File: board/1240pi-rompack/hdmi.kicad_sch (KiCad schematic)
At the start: 3 parts, among them J2 RaspberryPi_CM4_B, J3 HDMI_A, J4 HDMI_A

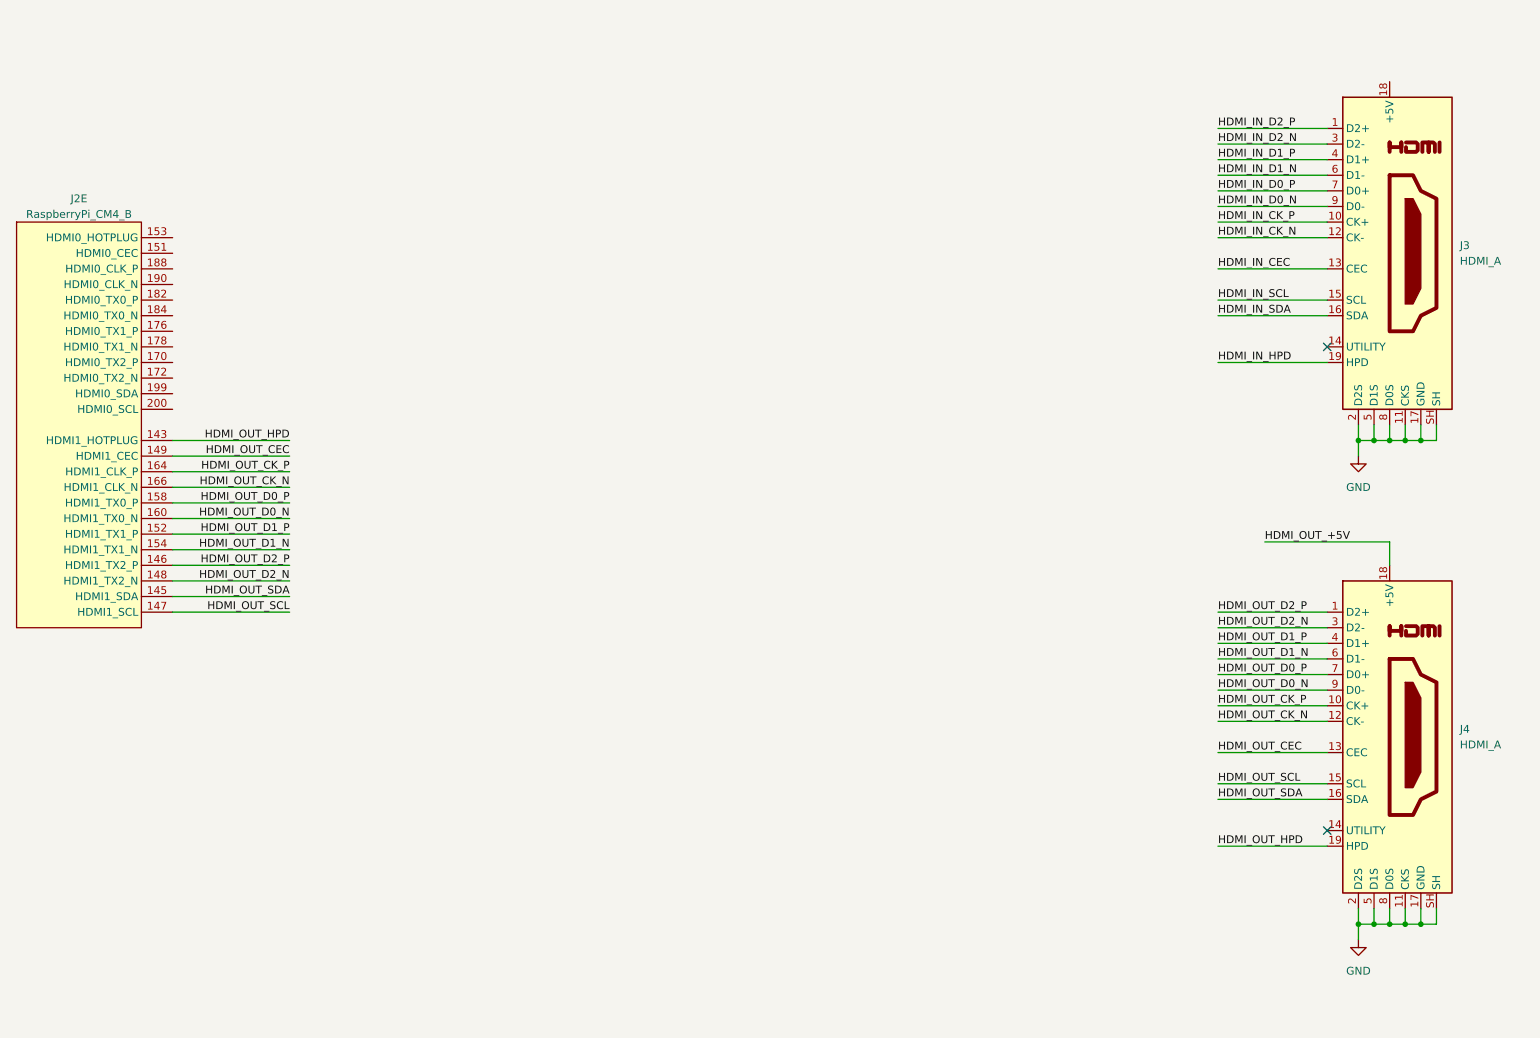
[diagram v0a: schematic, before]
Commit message: Route HDMI output port.
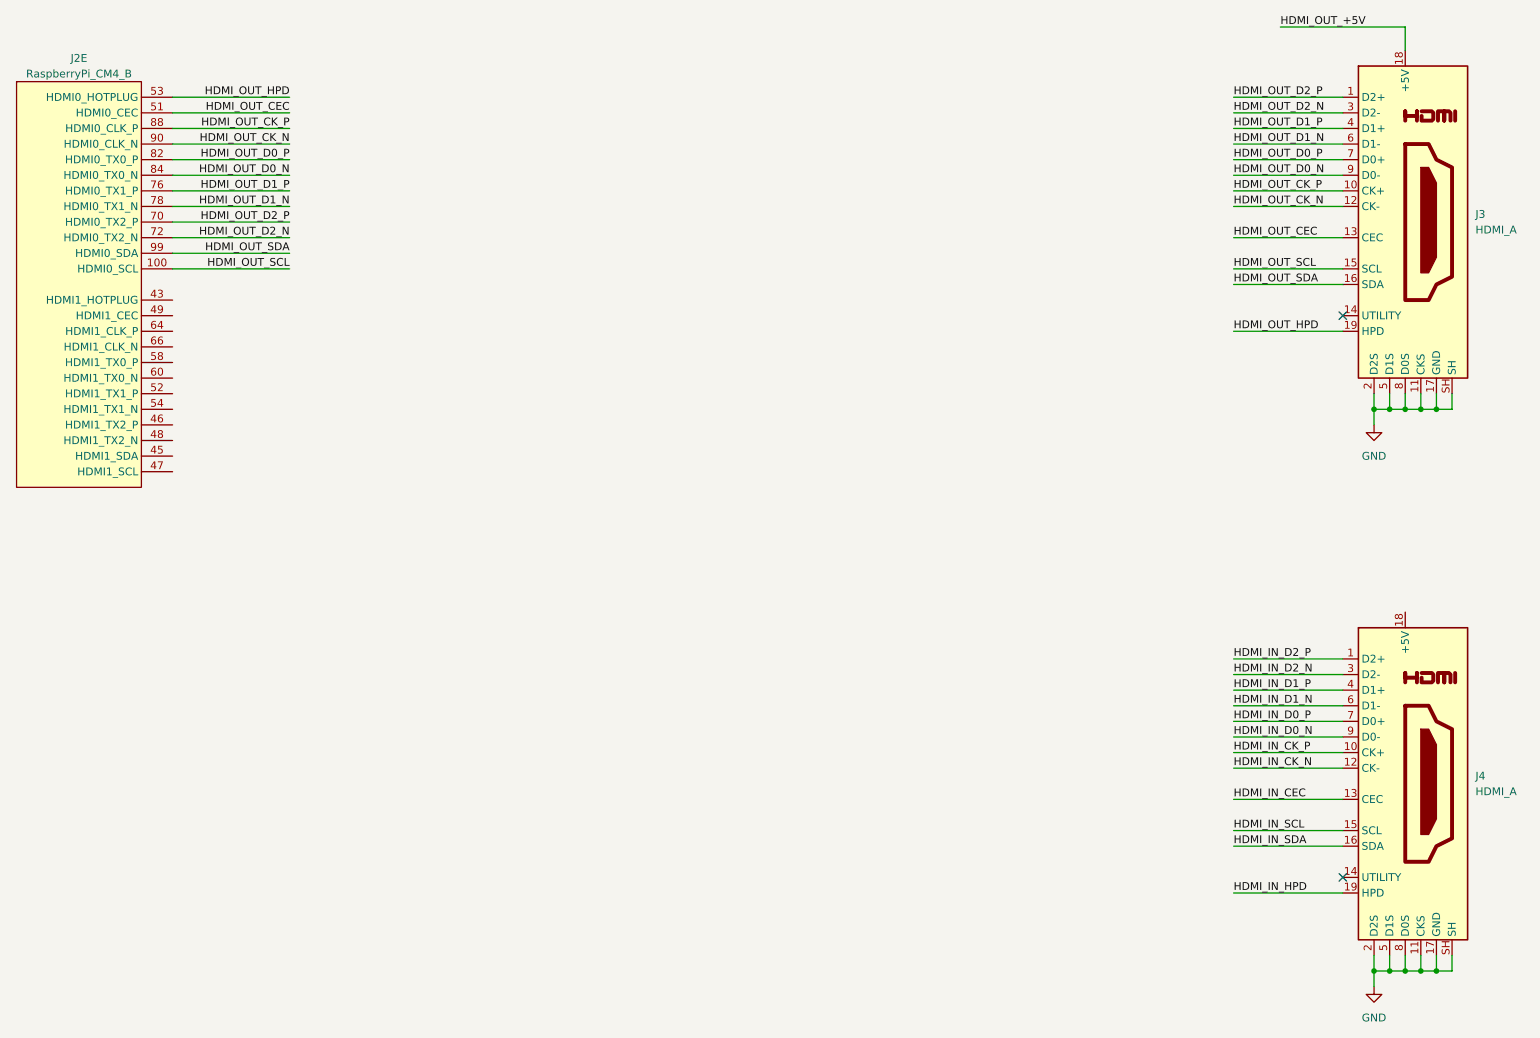
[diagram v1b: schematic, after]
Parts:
- renumbered J4 to J3, J3 to J4
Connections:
- net HDMI_OUT_CEC: now also J2.51 (HDMI0_CEC); no longer J2.149 (HDMI1_CEC)
- net HDMI_OUT_CK_N: now also J2.90 (HDMI0_CLK_N); no longer J2.166 (HDMI1_CLK_N)
- net HDMI_OUT_CK_P: now also J2.88 (HDMI0_CLK_P); no longer J2.164 (HDMI1_CLK_P)
- net HDMI_OUT_D0_N: now also J2.84 (HDMI0_TX0_N); no longer J2.160 (HDMI1_TX0_N)
- net HDMI_OUT_D0_P: now also J2.82 (HDMI0_TX0_P); no longer J2.158 (HDMI1_TX0_P)
- net HDMI_OUT_D1_N: now also J2.78 (HDMI0_TX1_N); no longer J2.154 (HDMI1_TX1_N)
- net HDMI_OUT_D1_P: now also J2.76 (HDMI0_TX1_P); no longer J2.152 (HDMI1_TX1_P)
- net HDMI_OUT_D2_N: now also J2.72 (HDMI0_TX2_N); no longer J2.148 (HDMI1_TX2_N)
- net HDMI_OUT_D2_P: now also J2.70 (HDMI0_TX2_P); no longer J2.146 (HDMI1_TX2_P)
- net HDMI_OUT_HPD: now also J2.53 (HDMI0_HOTPLUG); no longer J2.143 (HDMI1_HOTPLUG)
- net HDMI_OUT_SCL: now also J2.100 (HDMI0_SCL); no longer J2.147 (HDMI1_SCL)
- net HDMI_OUT_SDA: now also J2.99 (HDMI0_SDA); no longer J2.145 (HDMI1_SDA)
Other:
- moved on the sheet: J2E, J3, J4
